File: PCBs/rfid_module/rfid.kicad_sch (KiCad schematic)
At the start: 47 parts, among them IC201 TLV9004SIRTER, IC202 MAX9027EBT+T, Q201 DMN21D2UFB-7B, Q202 DMP21D5UFB4-7B, Q203 DMN21D2UFB-7B, Q204 DMN21D2UFB-7B

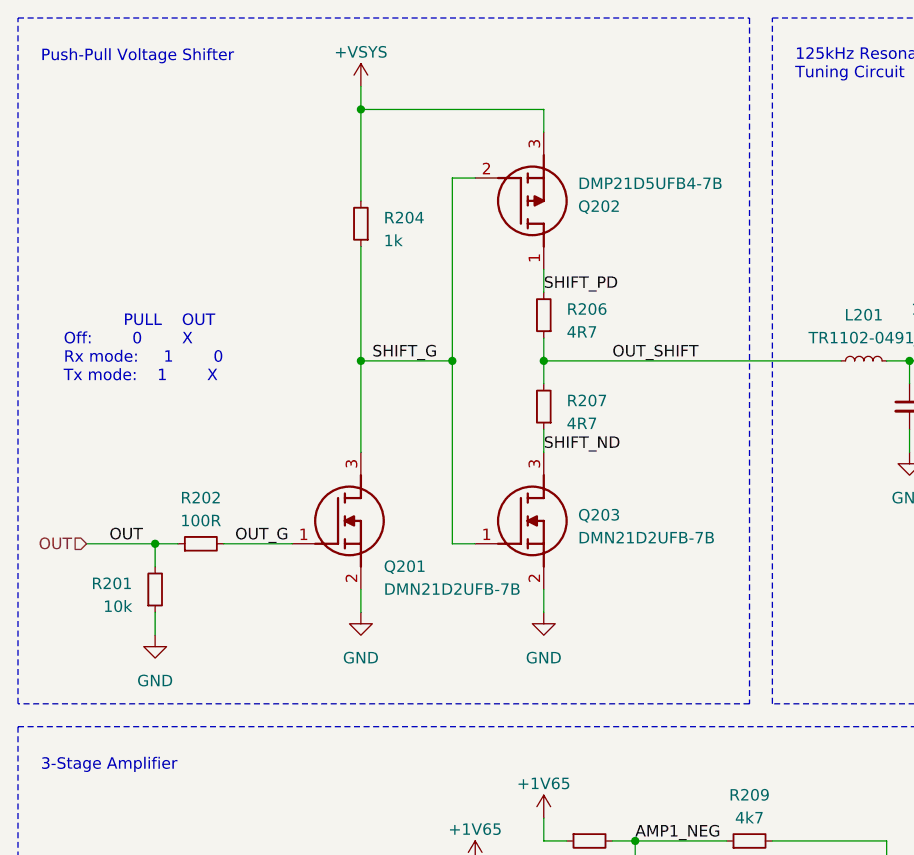
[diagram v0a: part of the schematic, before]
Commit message: RFID Module progress
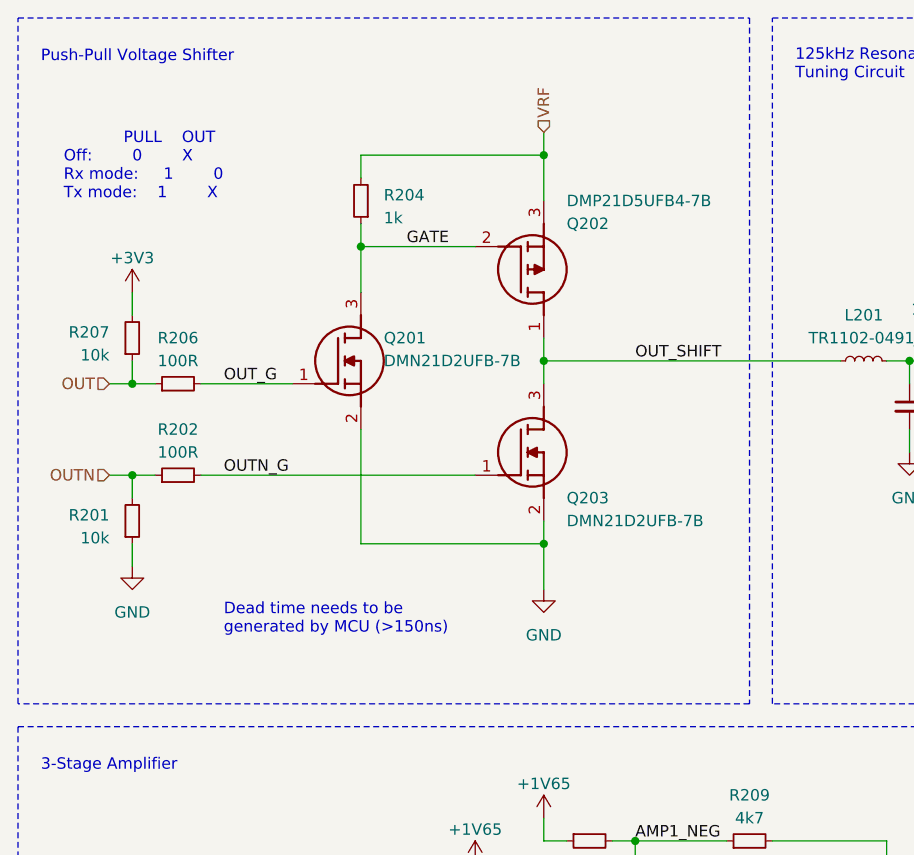
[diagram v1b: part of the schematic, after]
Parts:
- R206: value 4R7 -> 100R
- R207: value 4R7 -> 10k
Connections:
- net +3V3: now also R207.2
- net OUT: now also R206.1, R207.1; no longer R201.2, R202.1
- net OUT_G: now also R206.2; no longer R202.2
- net OUT_SHIFT: now also Q202.1 (D), Q203.3 (D); no longer R206.1, R207.2
- net +VSYS renamed VRF
- net SHIFT_G renamed GATE
- net GATE: no longer Q203.1 (G)
- removed net SHIFT_ND: Q203.3 (D), R207.1
- removed net SHIFT_PD: Q202.1 (D), R206.2
- new net OUTN: R201.2, R202.1
- new net OUTN_G: Q203.1 (G), R202.2
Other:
- note added: "Dead time needs to be generated by MCU (>150ns)"
- moved on the sheet: Q201, Q202, Q203, R204
